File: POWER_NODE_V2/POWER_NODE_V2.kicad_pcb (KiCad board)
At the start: 2 copper layers, 178 x 144 mm, 125 parts, among them J1 CONN_01X02, J10 CONN_02X07, J11 CONN_01X04, J12 CONN_01X04, J13 CONN_01X02, J14 CONN_01X02, J15 CONN_01X02, J16 CONN_01X03, J17 CONN_01X03, J18 CONN_01X03, J19 CONN_01X03, J2 CONN_01X02, J20 CONN_01X03, J21 CONN_01X03, J3 CONN_01X02, J4 CONN_01X02, J5 Booster_J1_J3, J6 I2C2_J10_8_9, J7 Booster_J4_J2, J8 CONN_01X01, J9 CONN_01X02, Q1 BSS84, Q2 BSS84, Q3 BSS84, Q4 BSS84, Q5 BSS84, Q6 BSS84, Q7 BSS84, U1 LM1117MP-3.3/NOPB, U10 DS2482S-100+T&R, U11 DS2482S-100+T&R, U12 NCV8405ADTRKG, U13 MAX14850AEE+, U14 MAX14850AEE+, U15 TL783CKTTR, U16 TL783CKTTR, U17 AMC1100DWV, U18 AMC1100DWV, U19 NUD3124LT1G, U2 R-745.0P, U20 RTE24024, U3 DS2482S-100+T&R, U4 DS2482S-100+T&R, U5 DS2482S-100+T&R, U6 TSYS01, U7 MS5607-02BA03, U8 DS2482S-100+T&R, U9 DS2482S-100+T&R

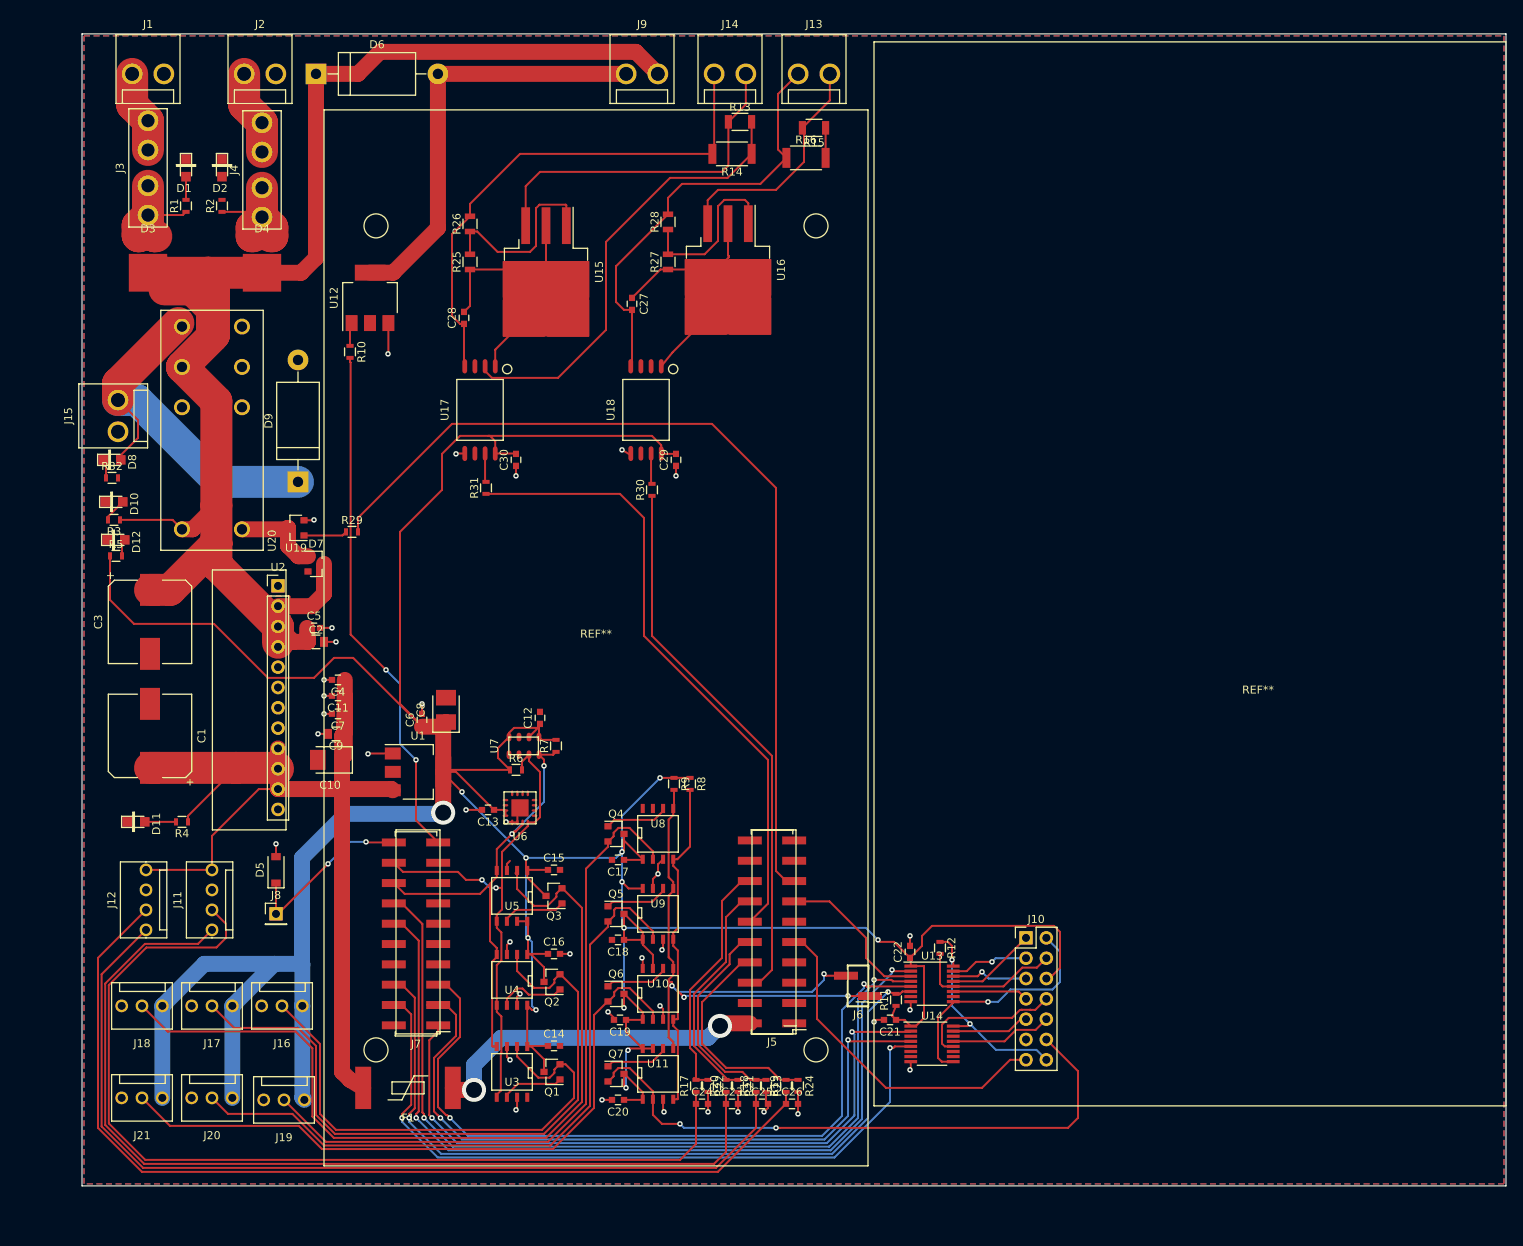
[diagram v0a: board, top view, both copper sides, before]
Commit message: Lot's of progress
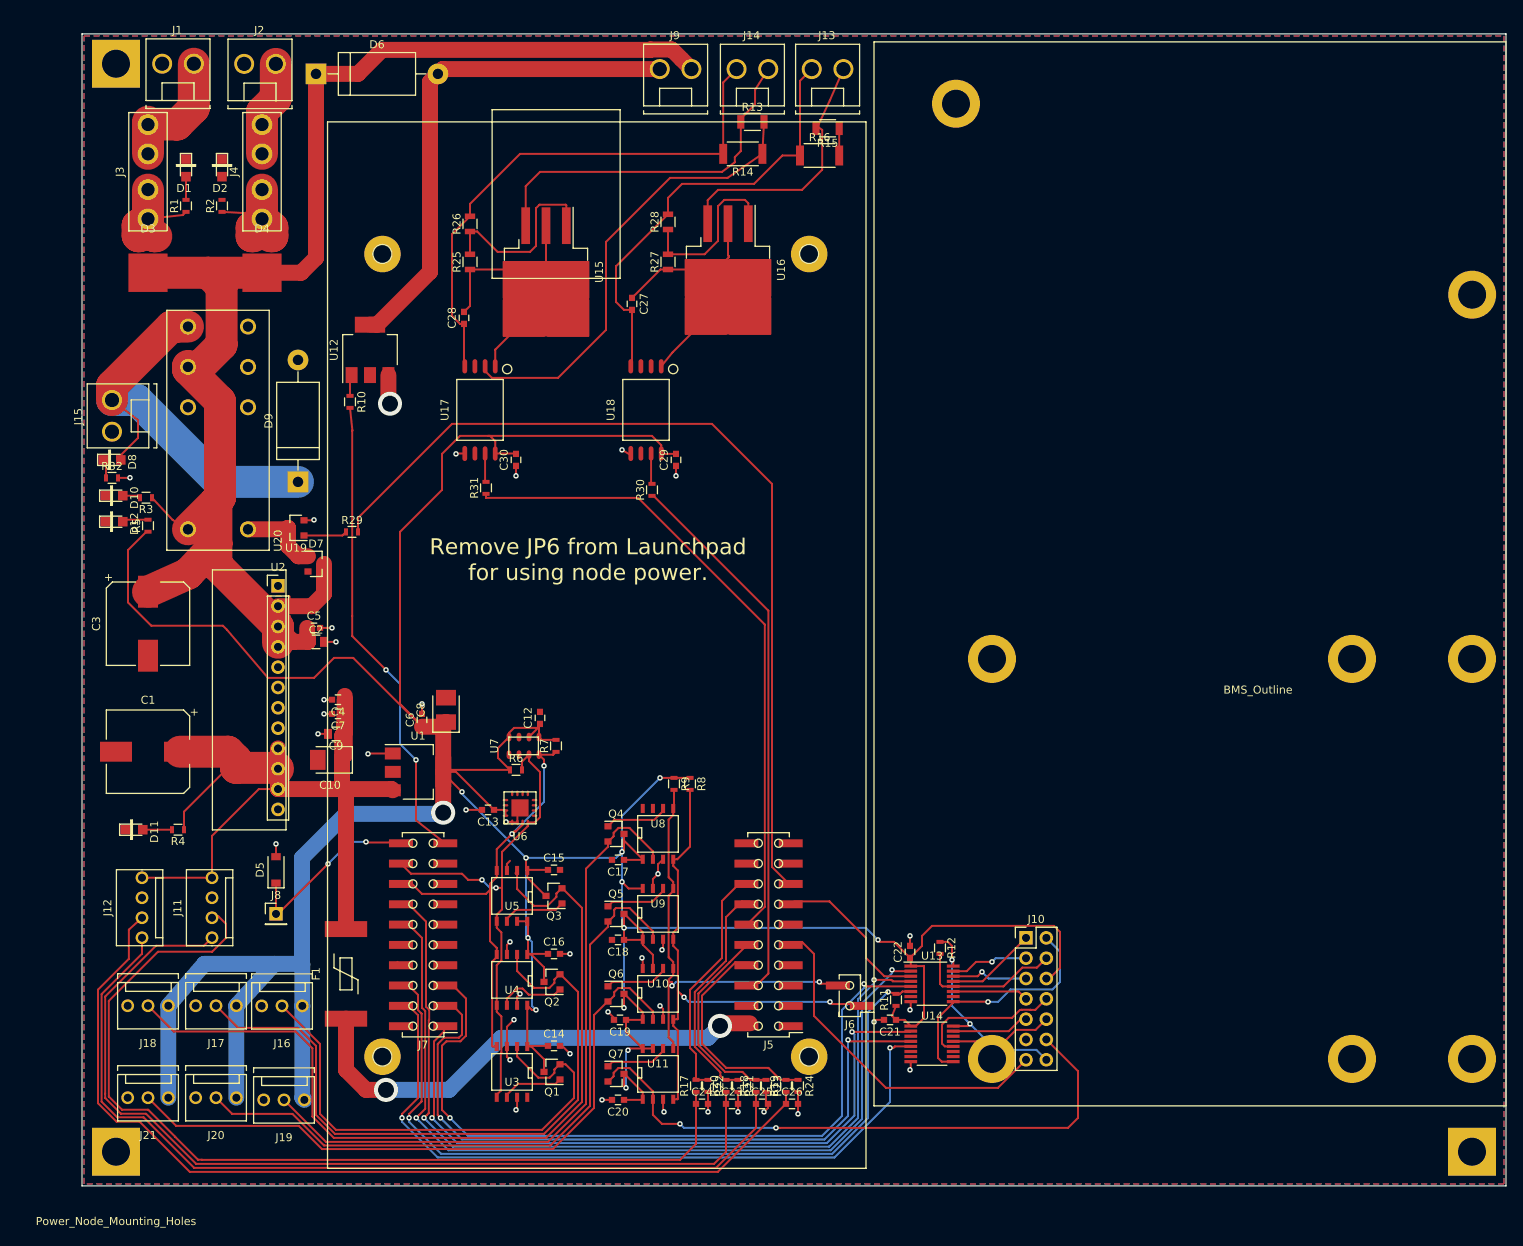
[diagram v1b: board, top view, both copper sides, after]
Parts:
- removed C11: 330uF / 35V / 20% / SMD 10x10, Capacitors_SMD:C_0603
- added Power_Node_Mounting_Holes: Power_Node_Mounting_Holes, rLoop_Footprints:Power_Node_Mounting_Holes, F.Cu at (33.2, 163.7)
- added RM57_Mounting_Holes: RM57_Mounting_Holes, rLoop_Footprints:RM57_Mounting_Hole, F.Cu at (66.6, 151.8)
- D1, D10, D11, D12, D2, D8: footprint rLoop Footprints:LED_0805 -> rLoop_Footprints:LED_0805
- D3, D4: value AS4PM-M3/86A -> FES10G; footprint rLoop Footprints:TO-277A_SMPC -> rLoop_Footprints:TO-277A_SMPC
- J1, J13, J14, J15, J2, J9: value CONN_01X02 -> TE_3-641119-2; footprint rLoop Footprints:TE_1744055-2_3.96_EP_HDR_ASSY_2P_VERT_HT -> rLoop_Footprints:3-641119-2_TE_2P_MTA156_HDR
- J16, J17, J18, J19, J20, J21: value CONN_01X03 -> 3-641215-3
- J3, J4: value CONN_01X02 -> Keystone_3544-2
- J5: value Booster_J1_J3 -> 5-146130-9; footprint rLoop Footprints:Booster1_Header_J1_J3 -> rLoop_Footprints:Booster1_Header_J1_J3
- J7: value Booster_J4_J2 -> 5-146130-9; footprint rLoop Footprints:Booster1_J4_J2 -> rLoop_Footprints:Booster1_J4_J2
- RM_57_Outline: renamed from REF**; footprint rLoop Footprints:RM57_Launchpad_Outline -> rLoop_Footprints:RM57_Launchpad_Outline
- U17, U18: footprint rLoop Footprints:amc1100_SOIC8 -> rLoop_Footprints:amc1100_SOIC8
- U6: footprint rLoop Footprints:QFN16_4x4 -> rLoop_Footprints:QFN16_4x4
- U7: footprint rLoop Footprints:ms5607-02ba03 -> rLoop_Footprints:ms5607-02ba03
- moved RM_57_Outline 72.8 mm to (127.0, 35.0)
- moved F1 16.2 mm to (62.0, 141.5), turned to 270 degrees
- moved U12 6.50 mm to (65.0, 63.5)
- moved R10 6.25 mm to (62.5, 70.0)
- moved R5 5.50 mm to (37.2, 85.5), turned to 90 degrees
- moved R3 4.87 mm to (37.0, 82.0)
- moved J9 4.24 mm to (103.2, 28.4)
- moved J1 3.96 mm to (41.0, 27.7)
- moved J14 2.86 mm to (112.8, 28.4)
- moved C4 2.48 mm to (61.0, 107.2)
- moved D12 2.28 mm to (33.0, 85.0)
- moved C1 2.00 mm to (37.2, 113.7), turned to 180 degrees
- moved J13 1.80 mm to (122.2, 28.4)
- moved R16 1.73 mm to (121.2, 39.2)
- moved R15 1.70 mm to (122.2, 35.8)
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- renumbered REF** to BMS_Outline
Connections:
- J13 pad 1: CHARGE_P_HOT -> CHARGE_N_HOT
- J13 pad 2: CHARGE_N_HOT -> CHARGE_P_HOT
- J14 pad 1: BATT_P_HOT -> BATT_N_HOT
- J14 pad 2: BATT_N_HOT -> BATT_P_HOT
- J15 pad 1: Net-(D8-Pad2) -> GND
- J15 pad 2: GND -> Net-(D8-Pad2)
- J9 pad 1: +24V -> Net-(D6-Pad2)
- J9 pad 2: Net-(D6-Pad2) -> +24V
- U17 pad 2: Net-(R13-Pad2) -> BATT_N_HOT
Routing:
- net BATT_N_HOT: track 65.3 -> 115.8 mm
- net Net-(R13-Pad2): track 56.3 -> 9.29 mm
- net +5V: track 131.1 -> 109.2 mm
- net Net-(F1-Pad2): track 42.5 -> 61.4 mm
- net +24V: track 199.7 -> 187.5 mm
- net Net-(D6-Pad2): track 53.6 -> 63.4 mm
- net Net-(J1-Pad2): track 10.3 -> 16.1 mm
- net /BMS Interface/BMS_FAN: track 65.1 -> 59.4 mm
- net GND: track 66.5 -> 72.2 mm, vias 37 -> 39
- net +3V3: track 529.8 -> 534.8 mm
- net Net-(C24-Pad1): track 121.2 -> 117.8 mm
- net Net-(C23-Pad1): track 121.5 -> 118.2 mm
- net CHARGE_P_HOT: track 29.3 -> 32.4 mm
- net Net-(C25-Pad1): track 117.7 -> 114.7 mm
- net Net-(C26-Pad1): track 123.0 -> 120.1 mm
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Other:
- board text added: "Remove JP6 from Launchpad for using node power."
- board text added: "Use No. 2 or M2 screws for mounting RM57."
